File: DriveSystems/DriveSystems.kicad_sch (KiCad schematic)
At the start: 12 parts, among them J1 Raspberry_Pi_4, U1 RoboClaw Motor Controller, U2 5304 Gear Motor, U3 24VDC UBC-C PSU

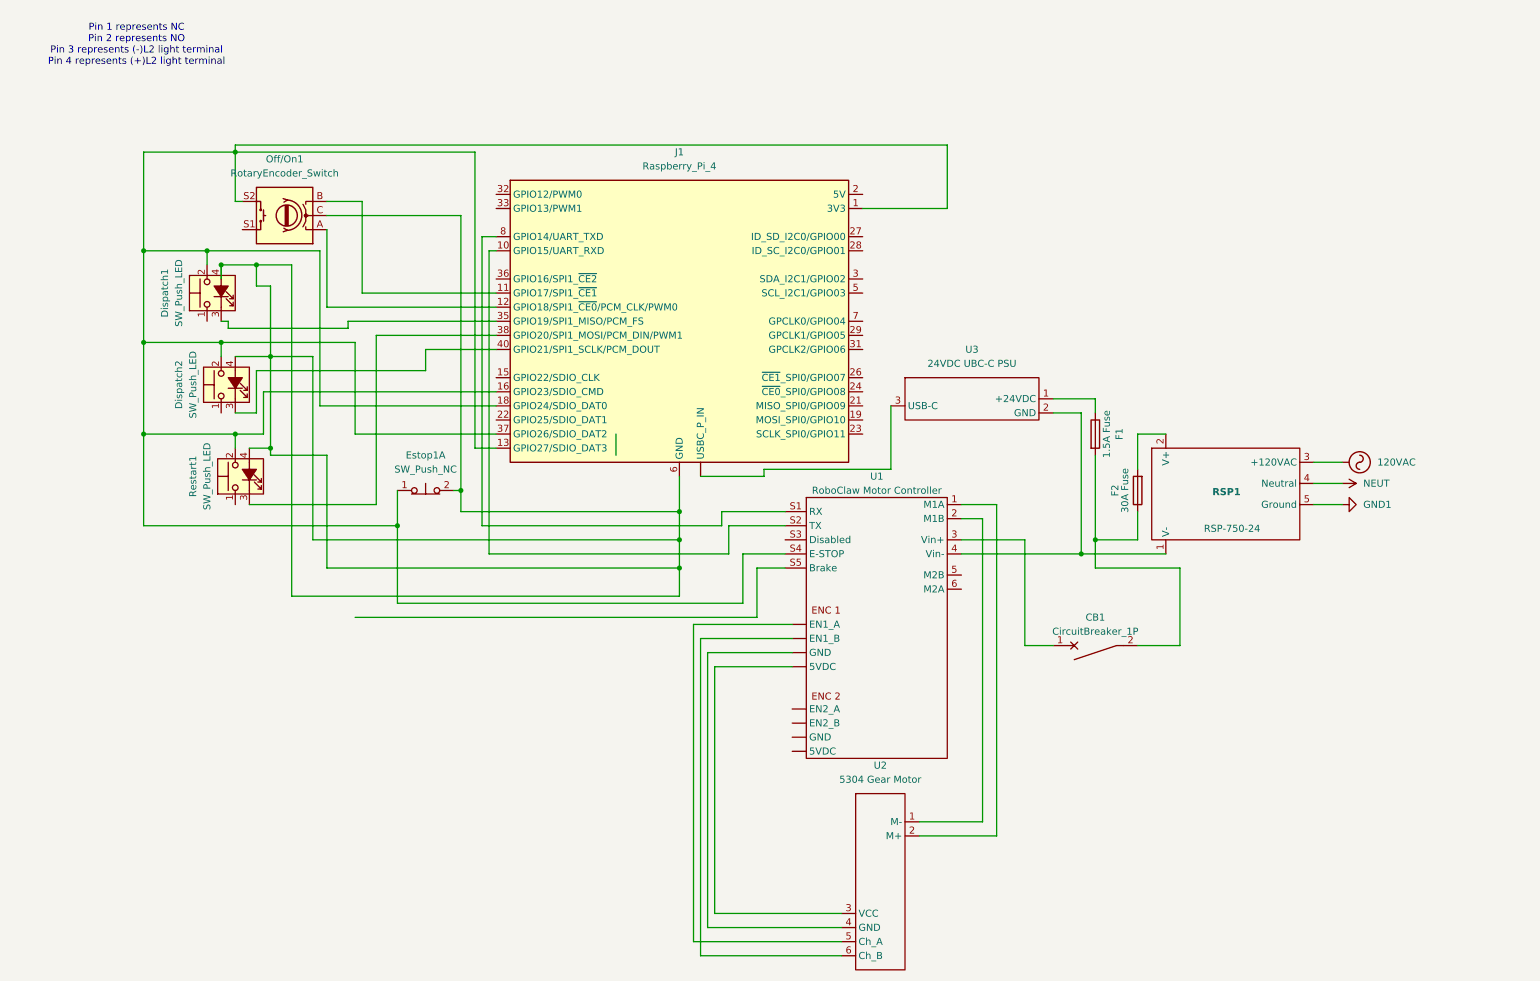
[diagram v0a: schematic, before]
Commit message: Cleanup & New things
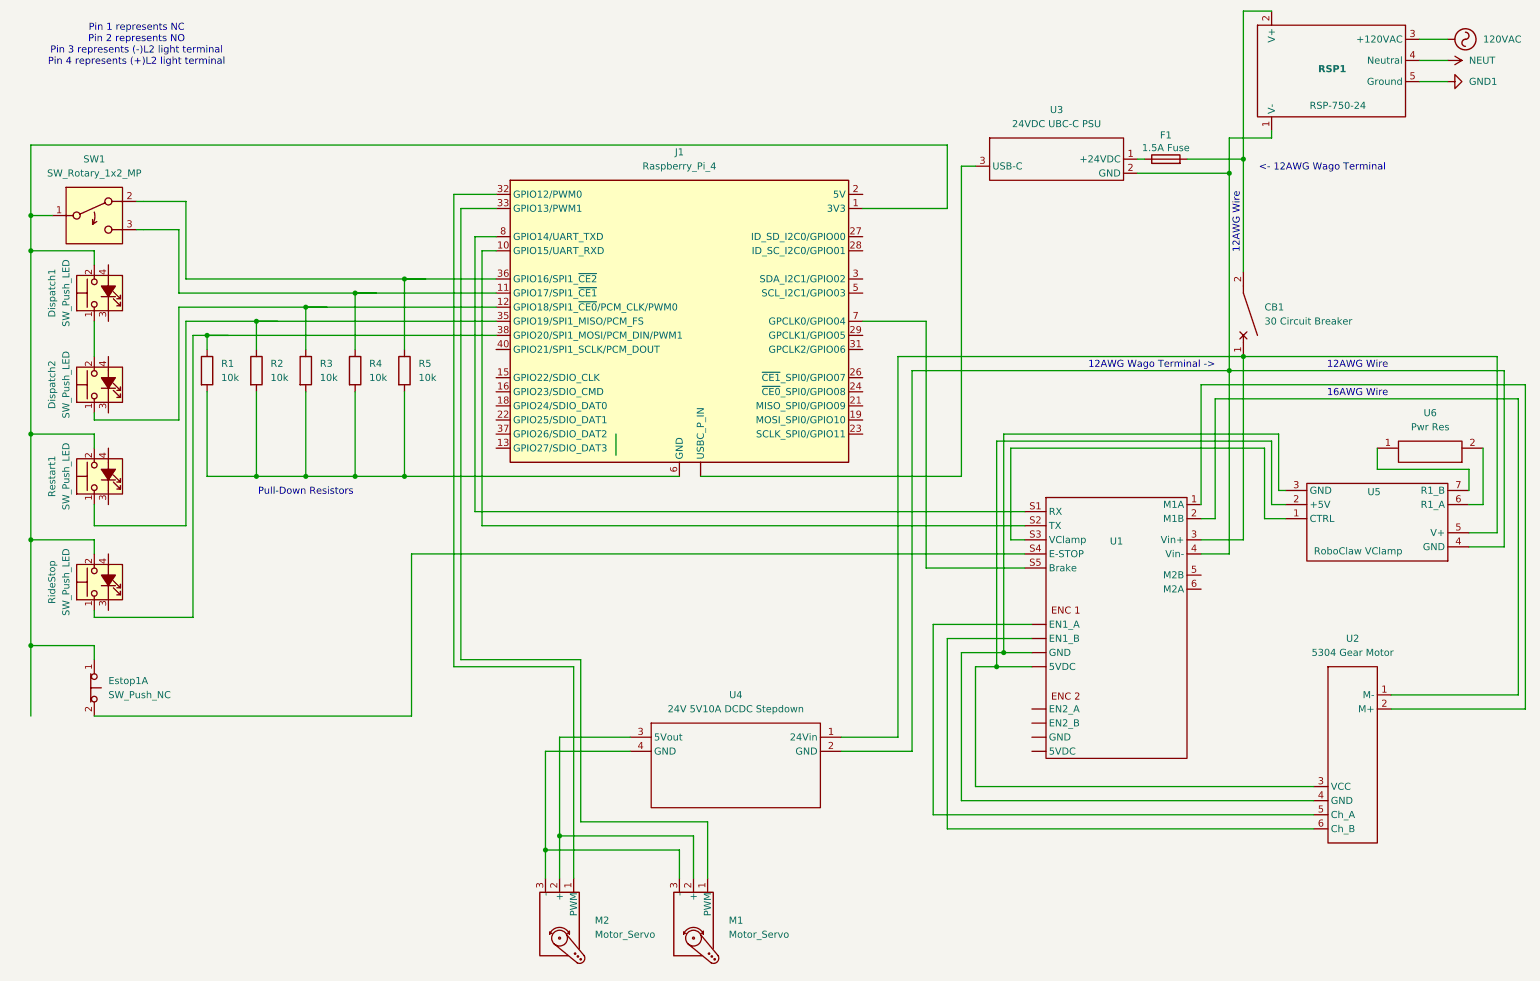
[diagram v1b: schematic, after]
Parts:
- removed F2: 30A Fuse, symbol Device:Fuse
- removed Off/On1: RotaryEncoder_Switch, symbol Device:RotaryEncoder_Switch
- added M1, M2: Motor_Servo, symbol Motor:Motor_Servo
- added R1, R2, R3, R4, R5: 10k, symbol Device:R
- added RideStop: SW_Push_LED, symbol Switch:SW_Push_LED
- added SW1: SW_Rotary_1x2_MP, symbol Switch:SW_Rotary_1x3_MP
- added U4: 24V 5V10A DCDC Stepdown, symbol CustomSymbols:24V 5V10A_DCDC_Stepdown
- added U5: RoboClaw VClamp, symbol CustomSymbols:RoboclawVClamp
- added U6: Pwr Res, symbol CustomSymbols:Power_Resistor
- CB1: value CircuitBreaker_1P -> 30 Circuit Breaker
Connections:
- net at J1.11 (GPIO17/SPI1_~{CE1}): now also R4.1, SW1.3
- net at J1.12 (GPIO18/SPI1_~{CE0}/PCM_CLK/PWM0): now also Dispatch2.1, R3.1
- net at J1.14 (GND), J1.20 (GND), J1.25 (GND)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: now also R1.2, R2.2, R3.2, R4.2, R5.2; no longer Dispatch1.4 (A), Dispatch2.4 (A), Estop1.2, Restart1.4 (A)
- net at J1.32 (GPIO12/PWM0): now also M2.1 (PWM)
- net at J1.33 (GPIO13/PWM1): now also M1.1 (PWM)
- net at J1.35 (GPIO19/SPI1_MISO/PCM_FS): now also Restart1.1, R2.1; no longer Dispatch1.3 (K)
- net at J1.36 (GPIO16/SPI1_~{CE2}): now also R5.1, SW1.2
- net at J1.38 (GPIO20/SPI1_MOSI/PCM_DIN/PWM1): now also R1.1, RideStop.1; no longer Restart1.3 (K)
- net at J1.40 (GPIO21/SPI1_SCLK/PCM_DOUT): no longer Dispatch2.3 (K)
- net at J1.7 (GPCLK0/GPIO04): now also U1.S5 (Brake)
- net at U1. (5VDC): now also U2.6 (Ch_B)
- net at U1. (5VDC), U2.3 (VCC): now also U5.2 (+5V)
- net at U1. (5VDC), U2.4 (GND): now also U5.3 (GND)
- net at CB1.1, U1.3 (Vin+): now also U4.1 (24Vin), U5.5 (V+)
- net at U1.4 (Vin-), U3.2 (GND): now also U4.2 (GND), U5.4 (GND)
- net at U1.S3 (VClamp): now also U5.1 (CTRL)
- net at Dispatch1.1: now also Dispatch2.2
- new net: Dispatch1.2, Estop1.1, J1.1 (3V3), J1.17 (3V3), Restart1.2, RideStop.2, SW1.1
- new net: Estop1.2, U1.S4 (E-STOP)
- new net: M1.2 (+), M2.2 (+), U4.3 (5Vout)
- new net: M1.3 (-), M2.3 (-), U4.4 (GND)
- new net: U5.6 (R1_A), U6.2
- new net: U5.7 (R1_B), U6.1
- now unconnected: J1.13 (GPIO27/SDIO_DAT3), J1.16 (GPIO23/SDIO_CMD), J1.18 (GPIO24/SDIO_DAT0), J1.37 (GPIO26/SDIO_DAT2)
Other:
- note added: "12AWG Wago Terminal ->"
- note added: "12AWG Wire"
- note added: "16AWG Wire"
- note added: "<- 12AWG Wago Terminal"
- note added: "Pull-Down Resistors"
- moved on the sheet: CB1, Dispatch1, Dispatch2, Estop1A, F1, Restart1, U1, U2, U3
